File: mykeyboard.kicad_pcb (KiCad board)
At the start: 2 copper layers, 91.4 x 55.9 mm, 29 parts, among them J1 MJ-4PP-9, J2 LED, SW1 SW_PUSH, SW2 SW_PUSH, SW3 SW_PUSH, SW4 SW_PUSH, SW5 SW_PUSH, SW6 SW_PUSH, SW7 SW_PUSH, SW8 SW_PUSH, SW9 SW_PUSH, U1 ProMicro

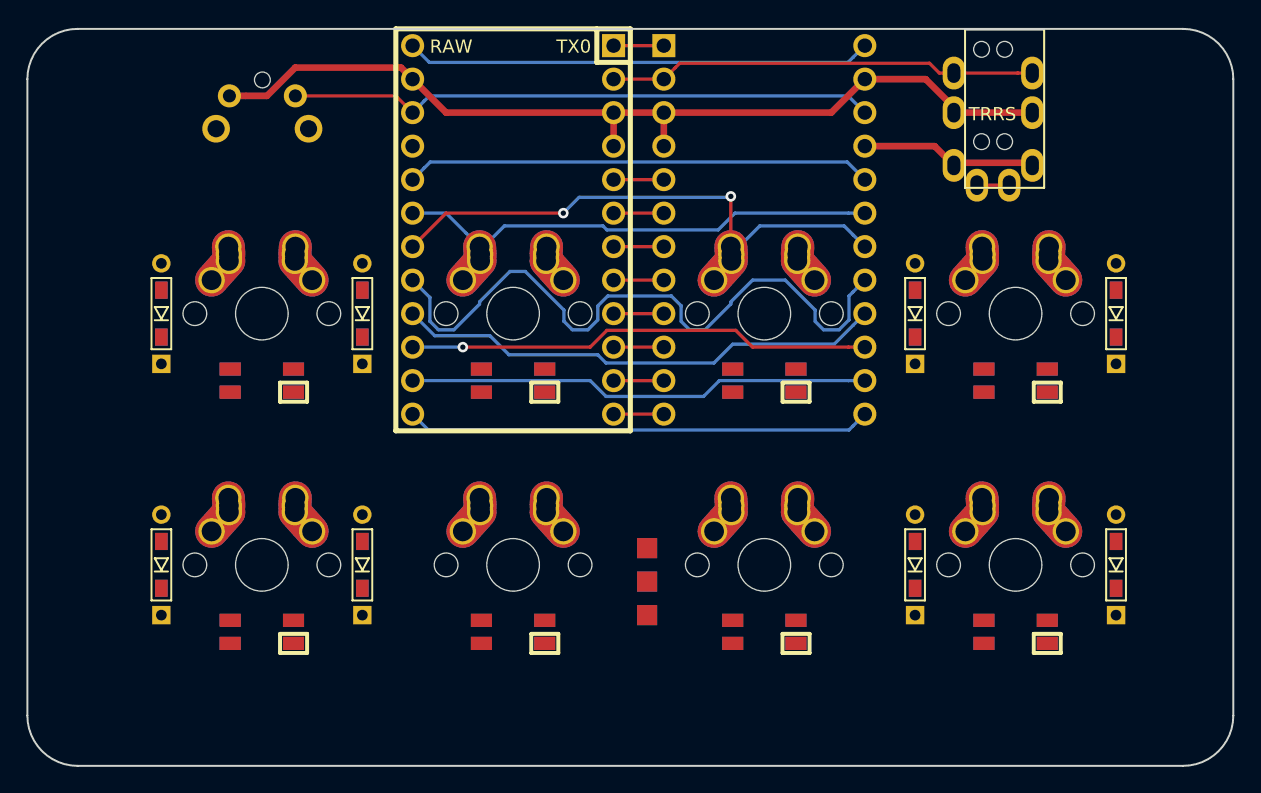
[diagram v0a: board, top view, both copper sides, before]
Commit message: 配線を済ませた
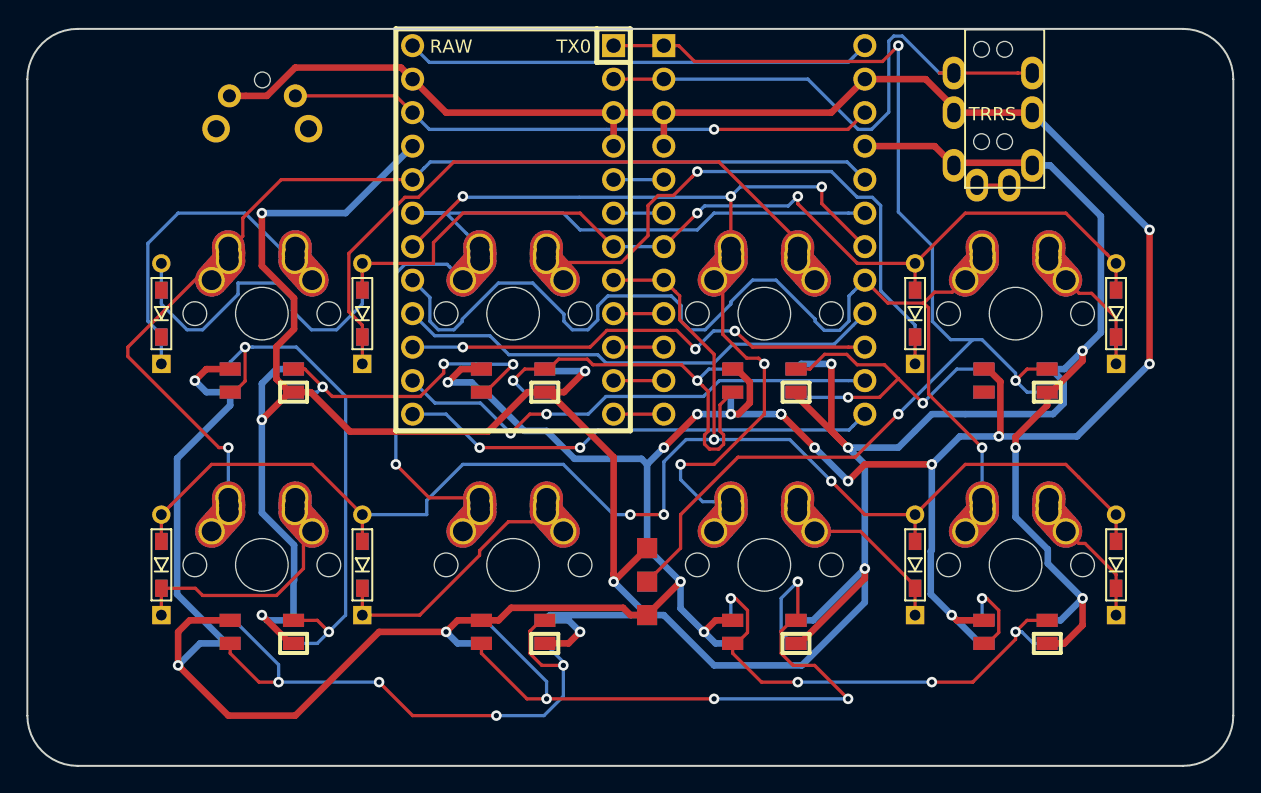
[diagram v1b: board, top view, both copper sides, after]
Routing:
- net VCC: track 13.5 -> 277.0 mm, vias 0 -> 12
- net GND: track 70.6 -> 297.2 mm, vias 0 -> 18
- net row1: track 3.81 -> 115.2 mm, vias 0 -> 5
- net row0: track 3.81 -> 101.0 mm, vias 0 -> 2
- net led: track 3.81 -> 92.4 mm, vias 0 -> 3
- net Net-(L4-Pad1): track 0.00 -> 56.7 mm, vias 0 -> 4
- net Net-(D5-Pad1): track 0.00 -> 49.7 mm
- net Net-(L2-Pad1): track 0.00 -> 45.6 mm, vias 0 -> 4
- net col0: track 35.4 -> 79.3 mm, vias 0 -> 1
- net Net-(D3-Pad1): track 0.00 -> 43.8 mm, vias 0 -> 1
- net Net-(L1-Pad1): track 0.00 -> 39.8 mm, vias 0 -> 2
- net Net-(L6-Pad1): track 0.00 -> 37.1 mm, vias 0 -> 4
- net Net-(L3-Pad3): track 0.00 -> 32.6 mm, vias 0 -> 2
- net col1: track 36.7 -> 69.2 mm, vias 0 -> 1
- net col2: track 41.2 -> 69.0 mm, vias 2 -> 5
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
